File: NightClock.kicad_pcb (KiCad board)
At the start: 2 copper layers, 196 x 90 mm, 0 parts

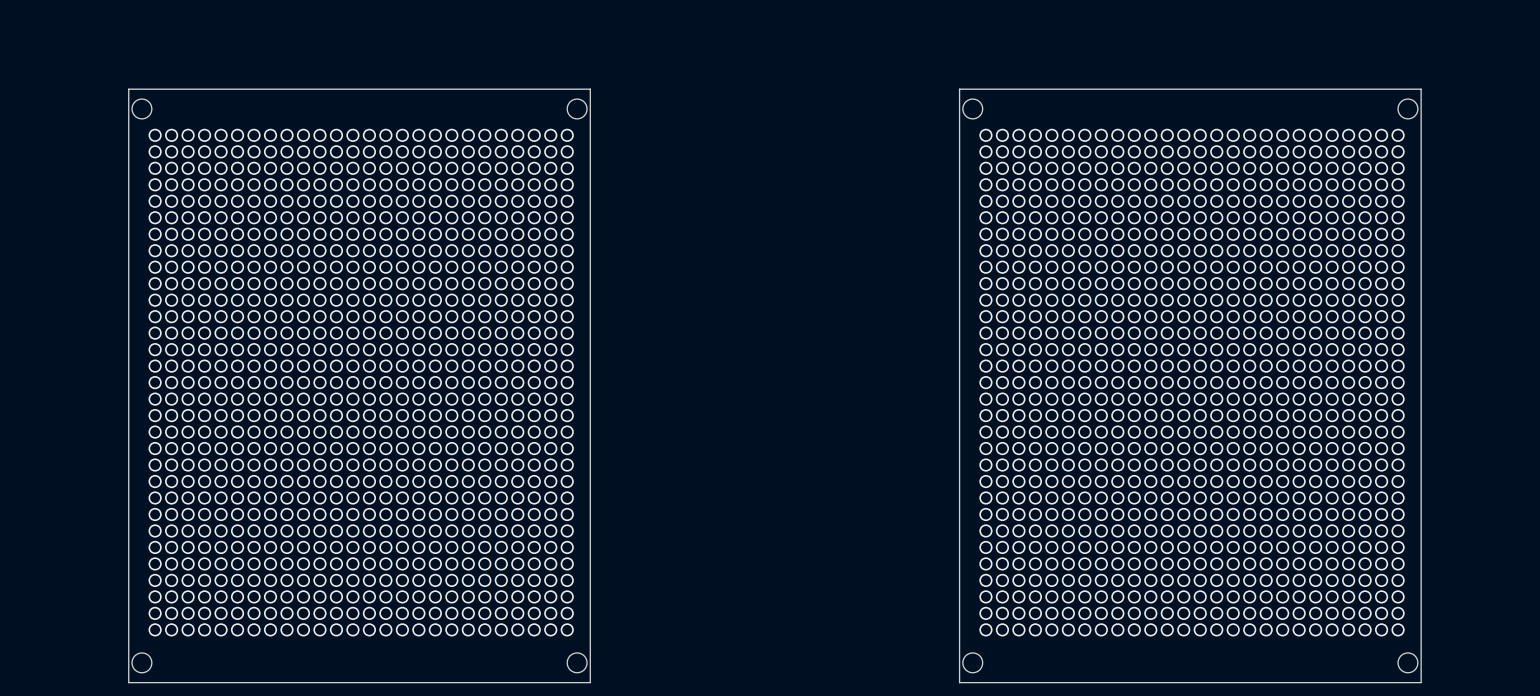
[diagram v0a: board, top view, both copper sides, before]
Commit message: make the pcb design
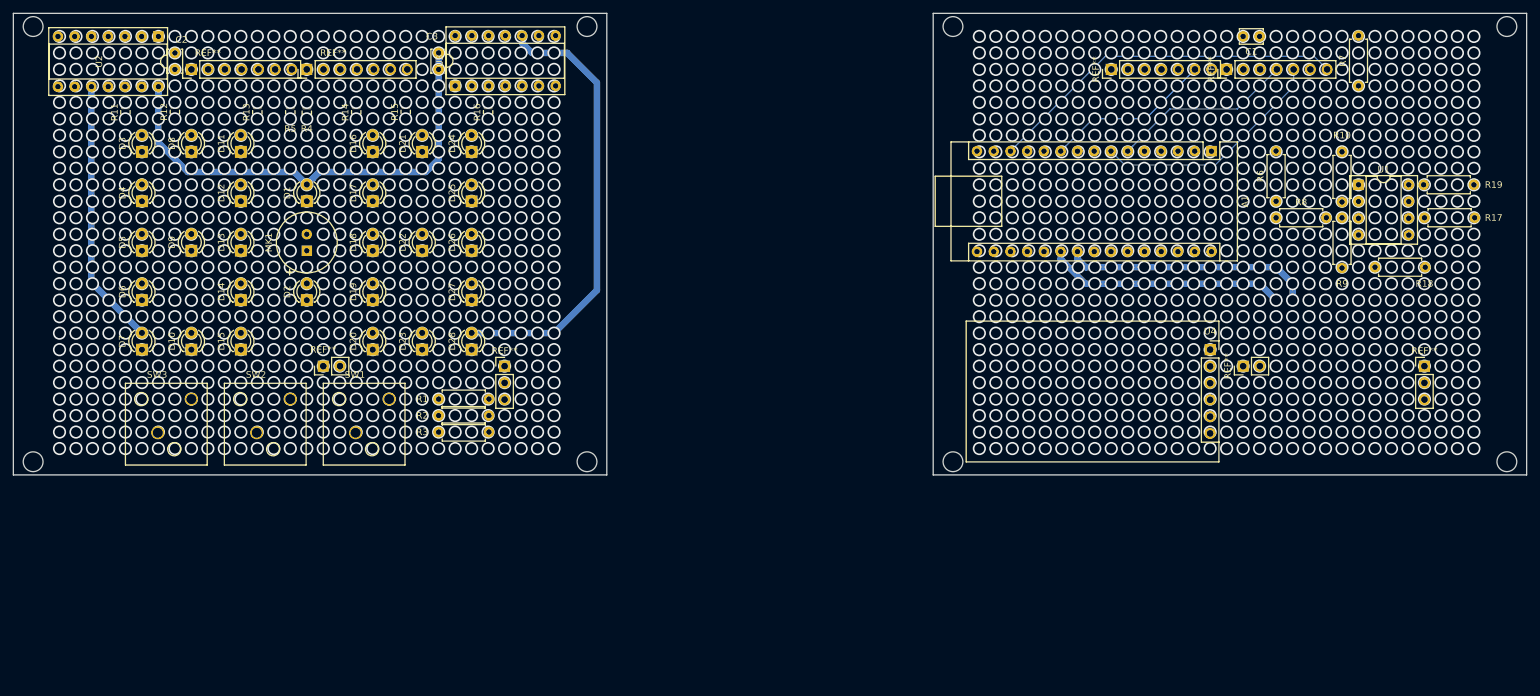
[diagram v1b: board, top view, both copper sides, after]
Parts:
- added A1: Arduino Nano, Module:Arduino_Nano, F.Cu at (212.2, 54.4)
- added C1: 100nF, Capacitor_THT:C_Disc_D3.4mm_W2.1mm_P2.50mm, F.Cu at (219.5, 37.0)
- added C2: 100nF, Capacitor_THT:C_Disc_D3.4mm_W2.1mm_P2.50mm, F.Cu at (55.0, 42.0)
- added C3: 100nF, Capacitor_THT:C_Disc_D3.4mm_W2.1mm_P2.50mm, F.Cu at (95.0, 39.5)
- added D1: LED, LED_THT:LED_D3.0mm, F.Cu at (75.0, 62.0)
- added D10: LED, LED_THT:LED_D3.0mm, F.Cu at (57.5, 84.5)
- added D11: LED, LED_THT:LED_D3.0mm, F.Cu at (65.0, 54.5)
- added D12: LED, LED_THT:LED_D3.0mm, F.Cu at (65.0, 62.0)
- added D13: LED, LED_THT:LED_D3.0mm, F.Cu at (65.0, 69.5)
- added D14: LED, LED_THT:LED_D3.0mm, F.Cu at (65.0, 77.0)
- added D15: LED, LED_THT:LED_D3.0mm, F.Cu at (65.0, 84.5)
- added D16: LED, LED_THT:LED_D3.0mm, F.Cu at (85.0, 54.5)
- added D17: LED, LED_THT:LED_D3.0mm, F.Cu at (85.0, 62.0)
- added D18: LED, LED_THT:LED_D3.0mm, F.Cu at (85.0, 69.5)
- added D19: LED, LED_THT:LED_D3.0mm, F.Cu at (85.0, 77.0)
- added D2: LED, LED_THT:LED_D3.0mm, F.Cu at (75.0, 77.0)
- added D20: LED, LED_THT:LED_D3.0mm, F.Cu at (85.0, 84.5)
- added D21: LED, LED_THT:LED_D3.0mm, F.Cu at (92.5, 54.5)
- added D22: LED, LED_THT:LED_D3.0mm, F.Cu at (92.5, 69.5)
- added D23: LED, LED_THT:LED_D3.0mm, F.Cu at (92.5, 84.5)
- added D24: LED, LED_THT:LED_D3.0mm, F.Cu at (100.0, 54.5)
- added D25: LED, LED_THT:LED_D3.0mm, F.Cu at (100.0, 62.0)
- added D26: LED, LED_THT:LED_D3.0mm, F.Cu at (100.0, 69.5)
- added D27: LED, LED_THT:LED_D3.0mm, F.Cu at (100.0, 77.0)
- added D28: LED, LED_THT:LED_D3.0mm, F.Cu at (100.0, 84.5)
- added D3: LED, LED_THT:LED_D3.0mm, F.Cu at (50.0, 54.5)
- added D4: LED, LED_THT:LED_D3.0mm, F.Cu at (50.0, 62.0)
- added D5: LED, LED_THT:LED_D3.0mm, F.Cu at (50.0, 69.5)
- added D6: LED, LED_THT:LED_D3.0mm, F.Cu at (50.0, 77.0)
- added D7: LED, LED_THT:LED_D3.0mm, F.Cu at (50.0, 84.5)
- added D8: LED, LED_THT:LED_D3.0mm, F.Cu at (57.5, 54.5)
- added D9: LED, LED_THT:LED_D3.0mm, F.Cu at (57.5, 69.5)
- added MK1: Microphone, Capacitor_THT:CP_Radial_Tantal_D9.0mm_P2.50mm, F.Cu at (75.0, 69.5)
- added R1: 1M, Resistor_THT:R_Axial_DIN0207_L6.3mm_D2.5mm_P7.62mm_Horizontal, F.Cu at (95.0, 92.0)
- added R10: 100k, Resistor_THT:R_Axial_DIN0207_L6.3mm_D2.5mm_P7.62mm_Horizontal, F.Cu at (232.0, 54.5)
- added R11: 150R, Resistor_SMD:R_0805_2012Metric, F.Cu at (47.5, 48.5)
- added R12: 150R, Resistor_SMD:R_0805_2012Metric, F.Cu at (55.0, 48.4)
- added R13: 150R, Resistor_SMD:R_0805_2012Metric, F.Cu at (67.5, 48.5)
- added R14: 150R, Resistor_SMD:R_0805_2012Metric, F.Cu at (82.5, 48.5)
- added R15: 150R, Resistor_SMD:R_0805_2012Metric, F.Cu at (90.0, 48.4)
- added R16: 150R, Resistor_SMD:R_0805_2012Metric, F.Cu at (102.5, 48.5)
- added R17: 100k, Resistor_THT:R_Axial_DIN0207_L6.3mm_D2.5mm_P7.62mm_Horizontal, F.Cu at (244.5, 64.5)
- added R18: 220k, Resistor_THT:R_Axial_DIN0207_L6.3mm_D2.5mm_P7.62mm_Horizontal, F.Cu at (237.0, 72.0)
- added R19: 22k, Resistor_THT:R_Axial_DIN0207_L6.3mm_D2.5mm_P7.62mm_Horizontal, F.Cu at (252.0, 59.5)
- added R2: 1M, Resistor_THT:R_Axial_DIN0207_L6.3mm_D2.5mm_P7.62mm_Horizontal, F.Cu at (95.0, 94.5)
- added R3: 1M, Resistor_THT:R_Axial_DIN0207_L6.3mm_D2.5mm_P7.62mm_Horizontal, F.Cu at (95.0, 97.0)
- added R4: 150R, Resistor_SMD:R_0805_2012Metric, F.Cu at (75.0, 48.6)
- added R5: 150R, Resistor_SMD:R_0805_2012Metric, F.Cu at (72.5, 48.5)
- added R6: 1k, Resistor_THT:R_Axial_DIN0207_L6.3mm_D2.5mm_P7.62mm_Horizontal, F.Cu at (222.0, 62.0)
- added R7: 1k, Resistor_THT:R_Axial_DIN0207_L6.3mm_D2.5mm_P7.62mm_Horizontal, F.Cu at (234.5, 44.5)
- added R8: 100k, Resistor_THT:R_Axial_DIN0207_L6.3mm_D2.5mm_P7.62mm_Horizontal, F.Cu at (222.0, 64.5)
- added R9: 100k, Resistor_THT:R_Axial_DIN0207_L6.3mm_D2.5mm_P7.62mm_Horizontal, F.Cu at (232.0, 64.5)
- added REF**: 7 pins, Connector_PinHeader_2.54mm:PinHeader_1x07_P2.54mm_Vertical, F.Cu at (197.0, 42.0)
- added REF**: 7 pins, Connector_PinHeader_2.54mm:PinHeader_1x07_P2.54mm_Vertical, F.Cu at (214.5, 42.0)
- added REF**: 7 pins, Connector_PinHeader_2.54mm:PinHeader_1x07_P2.54mm_Vertical, F.Cu at (75.0, 42.0)
- added REF**: 7 pins, Connector_PinHeader_2.54mm:PinHeader_1x07_P2.54mm_Vertical, F.Cu at (57.5, 42.0)
- added REF**: 2 pins, Connector_PinHeader_2.54mm:PinHeader_1x02_P2.54mm_Vertical, F.Cu at (217.0, 87.0)
- added REF**: 2 pins, Connector_PinHeader_2.54mm:PinHeader_1x02_P2.54mm_Vertical, F.Cu at (77.5, 87.0)
- added REF**: 3 pins, Connector_PinHeader_2.54mm:PinHeader_1x03_P2.54mm_Vertical, F.Cu at (244.5, 87.0)
- added REF**: 3 pins, Connector_PinHeader_2.54mm:PinHeader_1x03_P2.54mm_Vertical, F.Cu at (105.0, 87.0)
- added SW1: PUSH+, NightClockFootprints:PushButtonBlack, F.Cu at (87.5, 92.0)
- added SW2: PUSHOK, NightClockFootprints:PushButtonBlack, F.Cu at (72.5, 92.0)
- added SW3: PUSH-, NightClockFootprints:PushButtonBlack, F.Cu at (57.5, 92.0)
- added U1: TL082CP, Package_DIP:DIP-8_W7.62mm_Socket, F.Cu at (234.5, 59.5)
- added U2: 74HC164, Package_DIP:DIP-14_W7.62mm_Socket, F.Cu at (52.5, 37.0)
- added U3: 74HC164, Package_DIP:DIP-14_W7.62mm_Socket, F.Cu at (97.5, 44.5)
- added U4: DS3231Module, Connector_PinSocket_2.54mm:PinSocket_1x06_P2.54mm_Vertical, F.Cu at (212.0, 84.5)
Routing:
- net GND: track 0.00 -> 318.7 mm, vias 0 -> 84
- net +5V: track 0.00 -> 294.2 mm, vias 0 -> 82
- net BTN-: track 0.00 -> 153.9 mm, vias 0 -> 50
- net BTNOK: track 0.00 -> 110.3 mm, vias 0 -> 32
- net BTN+: track 0.00 -> 95.4 mm, vias 0 -> 23
- net DATA2: track 0.00 -> 85.4 mm, vias 0 -> 36
- net CLK2: track 0.00 -> 83.8 mm, vias 0 -> 4
- net MICINT: track 0.00 -> 83.4 mm, vias 0 -> 23
- net Net-(D20-Pad2): track 0.00 -> 83.2 mm, vias 0 -> 8
- net COLUMN1_2: track 0.00 -> 65.1 mm, vias 0 -> 28
- net MIC: track 0.00 -> 65.0 mm, vias 0 -> 27
- net Net-(D14-Pad2): track 0.00 -> 61.7 mm, vias 0 -> 8
- net DATA1: track 0.00 -> 60.5 mm, vias 0 -> 5
- net Net-(D13-Pad2): track 0.00 -> 59.1 mm, vias 0 -> 8
- net CLK1: track 0.00 -> 58.2 mm, vias 0 -> 4
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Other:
- board size 196 x 90 mm -> 229.5 x 70 mm
- copper layers 2 -> 4
- rule trace_min: 1 -> 0.2
- board text added: "BACK"
- board text added: "FRONT"
- board text added: "Vias: 2 mm 1.5 mm hole 31x26 Distance: 2.5 mm between vias Layers: Front - parts on the front Back - solid traces on the back Jump1, Jump2 - jumper cables"
- board text removed: "Vias: 2 mm 1.5 mm hole Distance: 2.5 mm between vias"
